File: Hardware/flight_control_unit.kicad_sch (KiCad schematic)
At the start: 43 parts, among them U14 STM32F405RGT6, U15 TDD01H0SB1R, U16 TDD01H0SB1R, Y2 25MHz

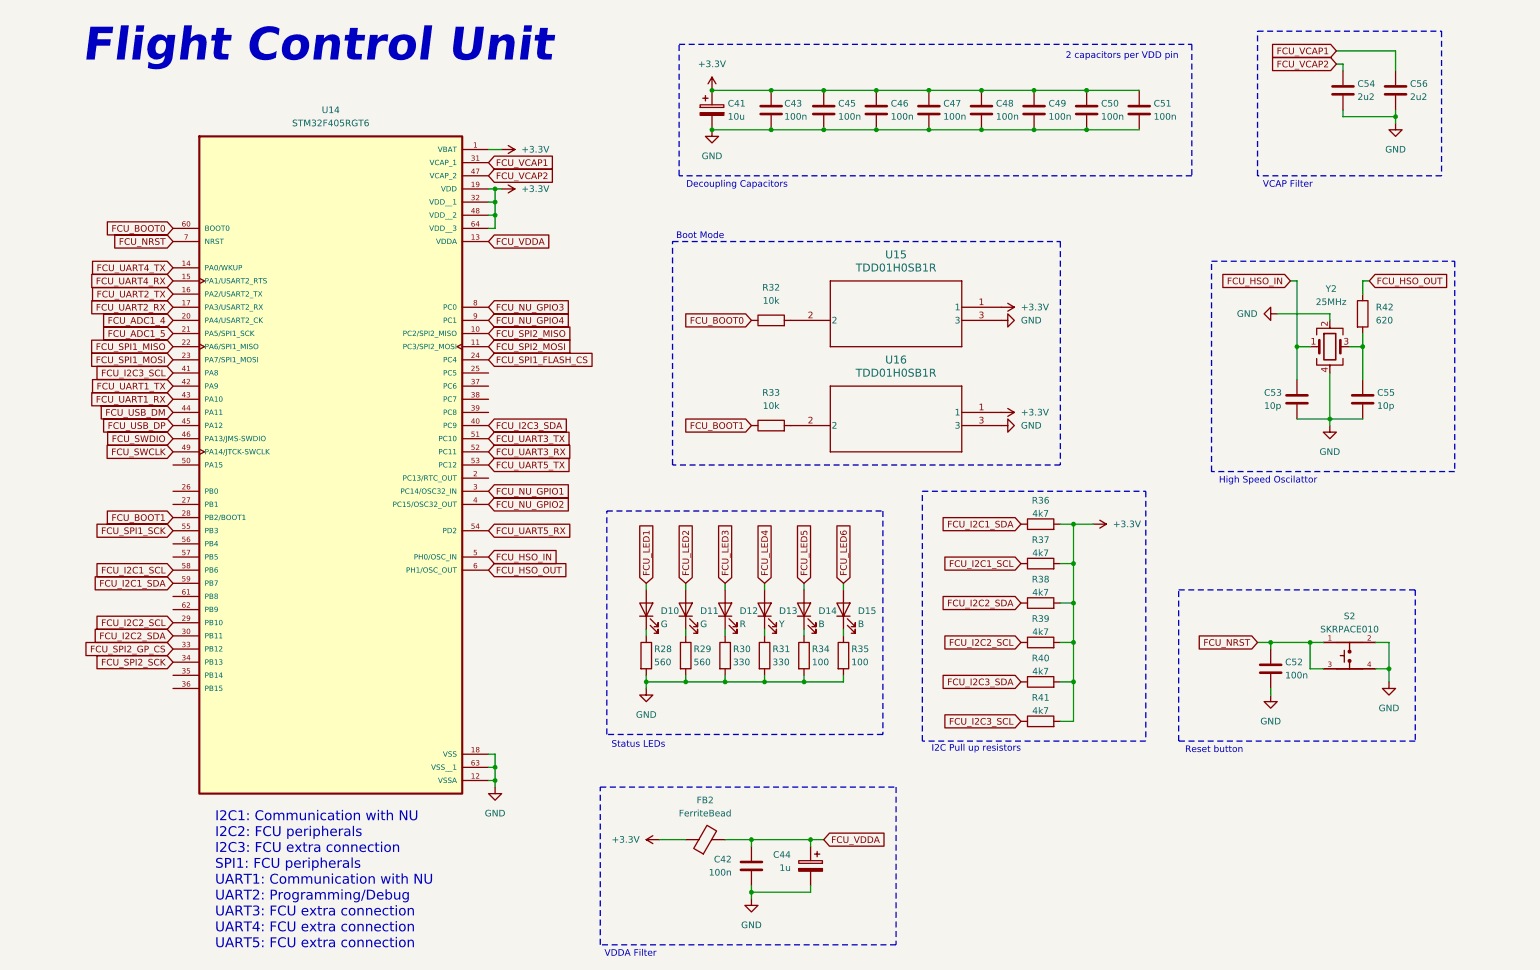
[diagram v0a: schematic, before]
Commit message: pin mess up win, starting over again
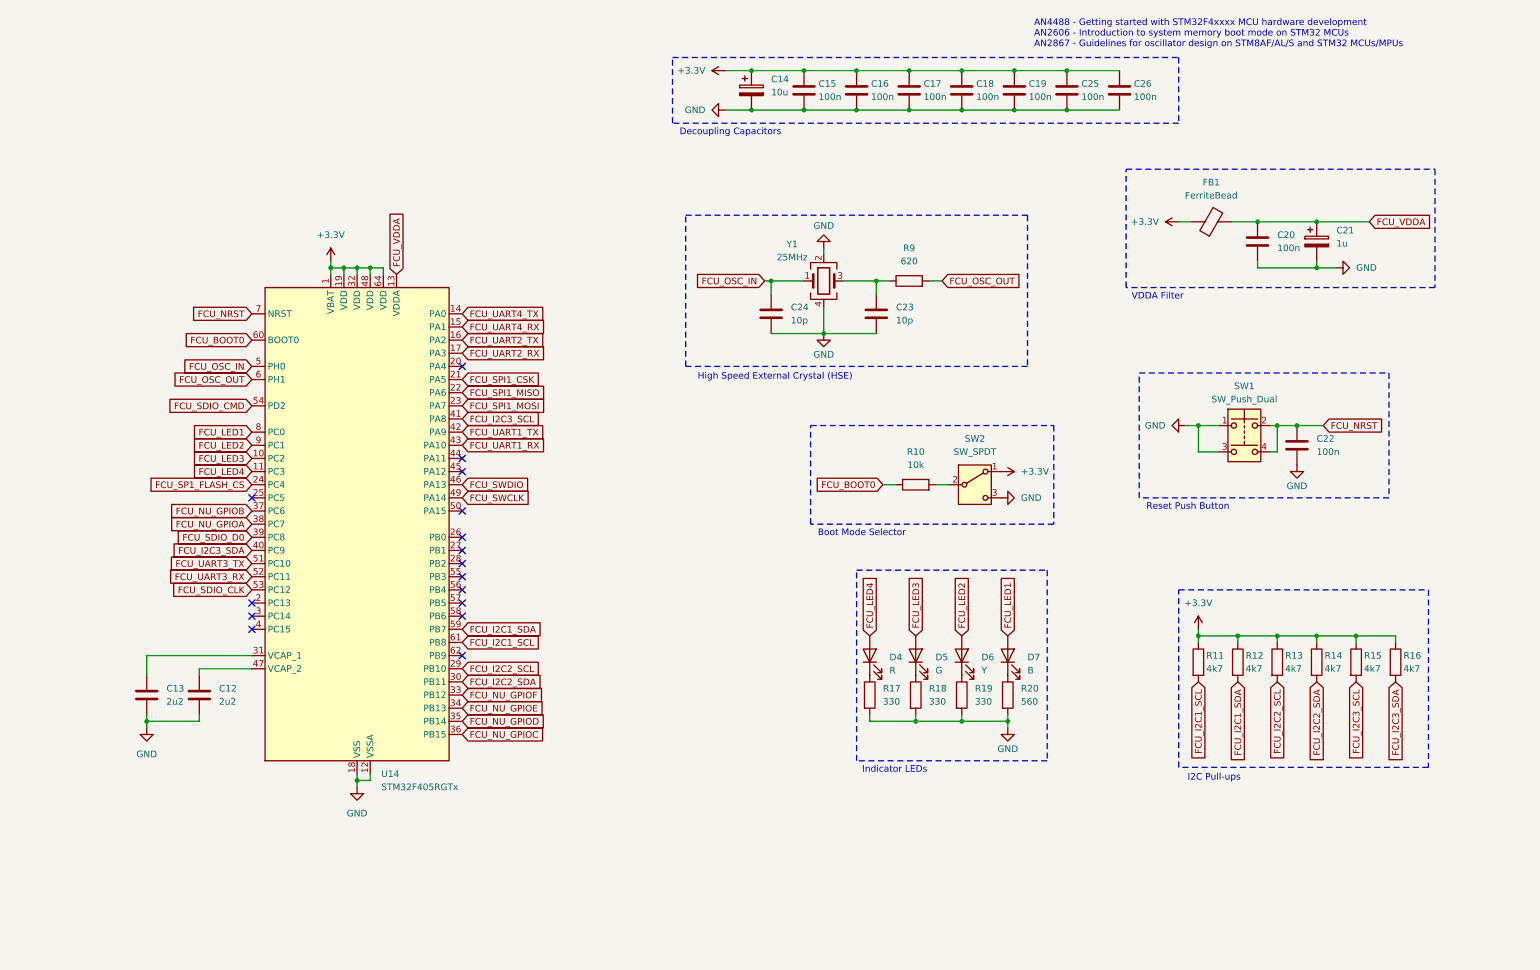
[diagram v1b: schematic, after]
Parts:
- removed C41: 10u, symbol Device:C_Polarized
- removed C42, C43, C45, C46, C47, C48, C49, C50, C51, C52: 100n, symbol Device:C
- removed C44: 1u, symbol Device:C_Polarized
- removed C53, C55: 10p, symbol Device:C
- removed C54, C56: 2u2, symbol Device:C
- removed D10, D11: G, symbol Device:LED
- removed D12: R, symbol Device:LED
- removed D13: Y, symbol Device:LED
- removed D14, D15: B, symbol Device:LED
- removed FB2: FerriteBead, symbol Device:FerriteBead
- removed R28, R29: 560, symbol Device:R
- removed R30, R31: 330, symbol Device:R
- removed R32, R33: 10k, symbol Device:R
- removed R34, R35: 100, symbol Device:R
- removed R36, R37, R38, R39, R40, R41: 4k7, symbol Device:R
- removed R42: 620, symbol Device:R
- removed S2: SKRPACE010, SKRPACE010:SW_SKRPACE010, symbol Aircraft_Components:SKRPACE010
- removed U14: STM32F405RGT6, STM32F405RGT6:QFP50P1200X1200X160-64N, symbol Aircraft_Components:STM32F405RGT6
- removed U15, U16: TDD01H0SB1R, SOT_TDDSB1R_CNK, symbol Aircraft_Components:TDD01H0SB1R
- removed Y2: 25MHz, symbol Device:Crystal_GND24
- added C12, C13: 2u2, symbol Device:C
- added C14: 10u, symbol Device:C_Polarized
- added C15, C16, C17, C18, C19, C20, C22, C25, C26: 100n, symbol Device:C
- added C21: 1u, symbol Device:C_Polarized
- added C23, C24: 10p, symbol Device:C
- added D4: R, symbol Device:LED
- added D5: G, symbol Device:LED
- added D6: Y, symbol Device:LED
- added D7: B, symbol Device:LED
- added FB1: FerriteBead, symbol Device:FerriteBead
- added R10: 10k, symbol Device:R
- added R11, R12, R13, R14, R15, R16: 4k7, symbol Device:R
- added R17, R18, R19: 330, symbol Device:R
- added R20: 560, symbol Device:R
- added R9: 620, symbol Device:R
- added SW1: SW_Push_Dual, symbol Switch:SW_Push_Dual
- added SW2: SW_SPDT, symbol Switch:SW_SPDT
- added U14: STM32F405RGTx, Package_QFP:LQFP-64_10x10mm_P0.5mm, symbol MCU_ST_STM32F4:STM32F405RGTx
- added Y1: 25MHz, symbol Device:Crystal_GND24
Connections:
- net +3.3V: now also C14.1, C15.1, C16.1, C17.1, C18.1, C19.1, C25.1, C26.1, FB1.1, R11.1, R12.1, R13.1, R14.1, R15.1, R16.1, SW2.1 (A), U14.1 (VBAT), U14.19 (VDD), U14.32 (VDD), U14.48 (VDD), U14.64 (VDD)
- net FCU_BOOT0: now also R10.1, U14.60 (BOOT0)
- net FCU_I2C1_SCL: now also R11.2, U14.61 (PB8)
- net FCU_I2C1_SDA: now also R12.2, U14.59 (PB7)
- net FCU_I2C2_SCL: now also R13.2, U14.29 (PB10)
- net FCU_I2C2_SDA: now also R14.2, U14.30 (PB11)
- net FCU_I2C3_SCL: now also R15.2, U14.41 (PA8)
- net FCU_I2C3_SDA: now also R16.2, U14.40 (PC9)
- net FCU_LED1: now also D7.2 (A), U14.8 (PC0)
- net FCU_LED2: now also D6.2 (A), U14.9 (PC1)
- net FCU_LED3: now also D5.2 (A), U14.10 (PC2)
- net FCU_LED4: now also D4.2 (A), U14.11 (PC3)
- net FCU_NRST: now also C22.1, SW1.2, SW1.4, U14.7 (NRST)
- net FCU_SPI1_MISO: now also U14.22 (PA6)
- net FCU_SPI1_MOSI: now also U14.23 (PA7)
- net FCU_SWCLK: now also U14.49 (PA14)
- net FCU_SWDIO: now also U14.46 (PA13)
- net FCU_UART1_RX: now also U14.43 (PA10)
- net FCU_UART1_TX: now also U14.42 (PA9)
- net FCU_UART2_RX: now also U14.17 (PA3)
- net FCU_UART2_TX: now also U14.16 (PA2)
- net FCU_UART3_RX: now also U14.52 (PC11)
- net FCU_UART3_TX: now also U14.51 (PC10)
- net FCU_UART4_RX: now also U14.15 (PA1)
- net FCU_UART4_TX: now also U14.14 (PA0)
- net FCU_VDDA: now also C20.1, C21.1, FB1.2, U14.13 (VDDA)
- net GND: now also C12.2, C13.2, C14.2, C15.2, C16.2, C17.2, C18.2, C19.2, C20.2, C21.2, C22.2, C23.2, C24.2, C25.2, C26.2, R17.2, R18.2, R19.2, R20.2, SW1.1, SW1.3, SW2.3 (C), U14.12 (VSSA), U14.18 (VSS), U14.63 (VSS), Y1.2, Y1.4
- new net: D7.1 (K), R20.1
- new net: R10.2, SW2.2 (B)
- new net: D6.1 (K), R19.1
- new net: D4.1 (K), R17.1
- new net: D5.1 (K), R18.1
- new net: C23.1, R9.1, Y1.3
- new net: C12.1, U14.47 (VCAP_2)
- new net: C13.1, U14.31 (VCAP_1)
- new net FCU_NU_GPIOA: U14.38 (PC7)
- new net FCU_NU_GPIOB: U14.37 (PC6)
- new net FCU_NU_GPIOC: U14.36 (PB15)
- new net FCU_NU_GPIOD: U14.35 (PB14)
- new net FCU_NU_GPIOE: U14.34 (PB13)
- new net FCU_NU_GPIOF: U14.33 (PB12)
- new net FCU_OSC_IN: C24.1, U14.5 (PH0), Y1.1
- new net FCU_OSC_OUT: R9.2, U14.6 (PH1)
- new net FCU_SDIO_CLK: U14.53 (PC12)
- new net FCU_SDIO_CMD: U14.54 (PD2)
- new net FCU_SDIO_D0: U14.39 (PC8)
- new net FCU_SP1_FLASH_CS: U14.24 (PC4)
- new net FCU_SPI1_CSK: U14.21 (PA5)
- no-connect marks 0 -> 16
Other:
- note added: "AN4488 - Getting started with STM32F4xxxx MCU hardware development AN2606 - Introduction to system memory boot mode on STM32 MCUs AN2867 - Guidelines for oscillator design on STM8AF/AL/S and STM32 MCUs/MPUs"
- note added: "Boot Mode Selector"
- note added: "High Speed External Crystal (HSE)"
- note added: "I2C Pull-ups"
- note added: "Indicator LEDs"
- note added: "Reset Push Button"
- note removed: "2 capacitors per VDD pin"
- note removed: "Boot Mode"
- note removed: "Flight Control Unit"
- note removed: "High Speed Oscilattor"
- note removed: "I2C Pull up resistors"
- note removed: "I2C1: Communication with NU I2C2: FCU peripherals I2C3: FCU extra connection SPI1: FCU peripherals UART1: Communication with NU UART2: Programming/Debug UART3: FCU extra connection UART4: FCU extra connection UART5: FCU extra connection"
- note removed: "Reset button"
- note removed: "Status LEDs"
- note removed: "VCAP Filter"
